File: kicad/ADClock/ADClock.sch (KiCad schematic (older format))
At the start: 26 parts, among them IC1 ATMEGA328-PU, IC2 ATMEGA328-PU, Y1 Crystal, Y2 Crystal

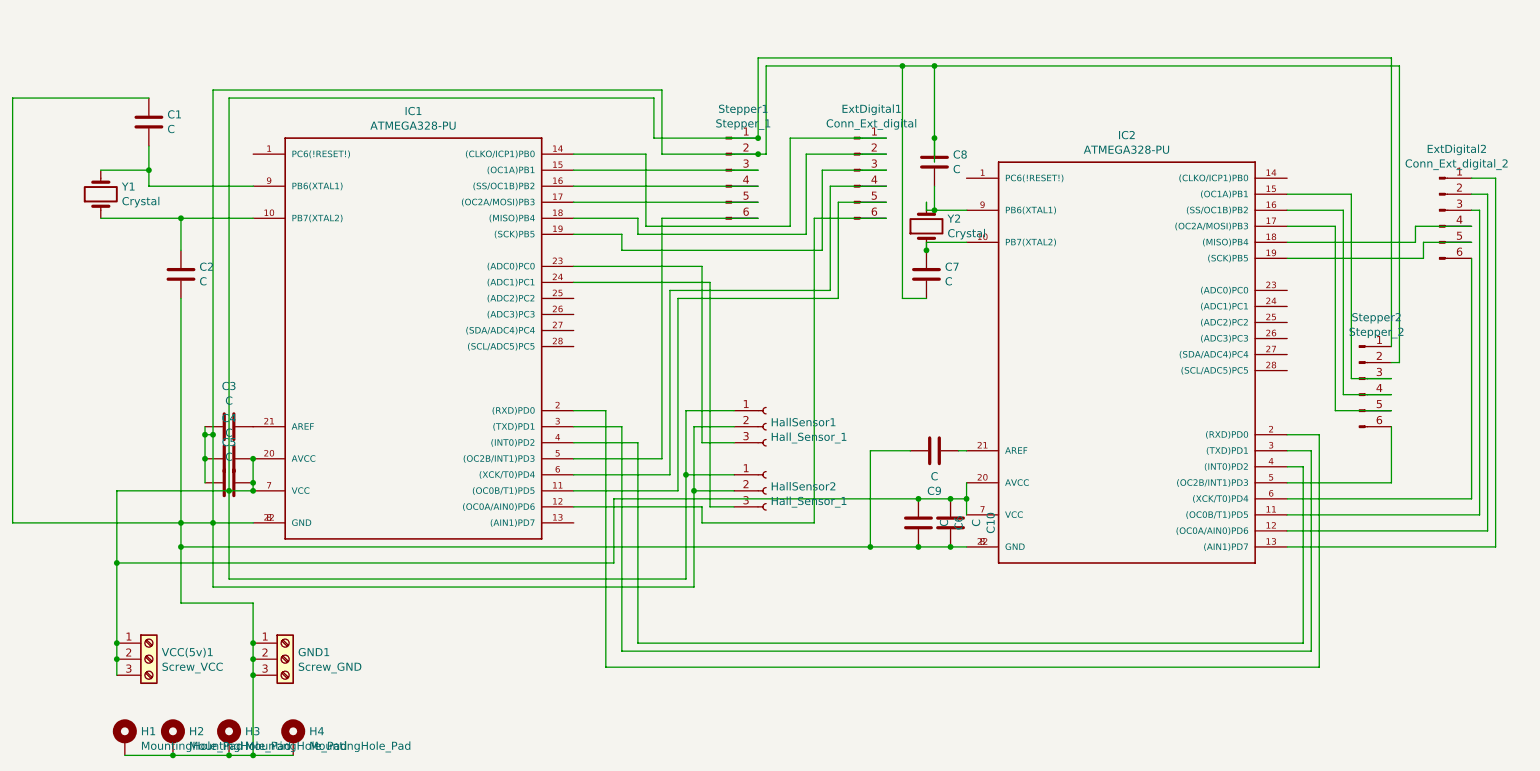
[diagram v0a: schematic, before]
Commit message: board changes
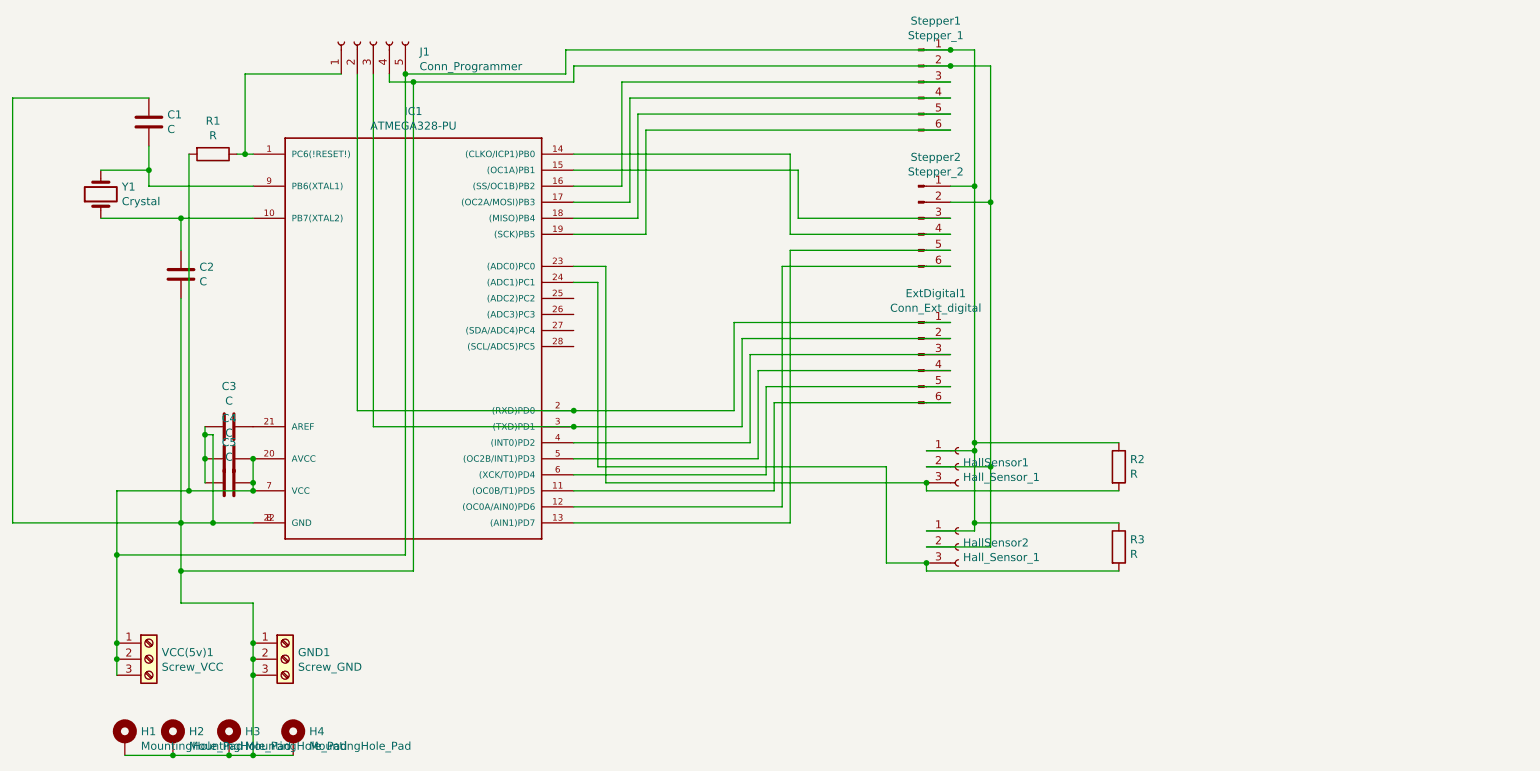
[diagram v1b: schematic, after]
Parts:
- removed C10, C6, C7, C8, C9: C, Capacitor_THT:C_Rect_L7.0mm_W2.5mm_P5.00mm, symbol Device:C
- removed ExtDigital2: Conn_Ext_digital_2, Connector_PinHeader_2.54mm:PinHeader_1x06_P2.54mm_Vertical, symbol Connector:Conn_01x06_Male
- removed IC2: ATMEGA328-PU, DIL28, symbol ATMEGA328-PU:ATMEGA328-PU
- removed Y2: Crystal, Crystal:Crystal_HC49-4H_Vertical, symbol Device:Crystal
- added J1: Conn_Programmer, Connector_PinHeader_2.54mm:PinHeader_1x05_P2.54mm_Vertical, symbol Connector:Conn_01x05_Female
- added R1, R2, R3: R, Resistor_THT:R_Axial_DIN0207_L6.3mm_D2.5mm_P7.62mm_Horizontal, symbol Device:R
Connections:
- net at C1.1, C2.2, C3.2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: now also J1.4 (Pin_4)
- net at IC1.1 (PC6(!RESET!)): now also J1.1 (Pin_1), R1.1
- net at IC1.11 ((OC0B/T1)PD5): now also ExtDigital1.6 (Pin_6); no longer ExtDigital1.5 (Pin_5)
- net at IC1.12 ((OC0A/AIN0)PD6): now also Stepper2.6 (Pin_6); no longer ExtDigital1.6 (Pin_6)
- net at IC1.13 ((AIN1)PD7): now also Stepper2.5 (Pin_5)
- net at IC1.14 ((CLKO/ICP1)PB0): now also Stepper2.4 (Pin_4); no longer ExtDigital1.1 (Pin_1)
- net at IC1.15 ((OC1A)PB1): now also Stepper2.3 (Pin_3); no longer Stepper1.3 (Pin_3)
- net at IC1.16 ((SS/OC1B)PB2): now also Stepper1.3 (Pin_3); no longer Stepper1.4 (Pin_4)
- net at IC1.17 ((OC2A/MOSI)PB3): now also Stepper1.4 (Pin_4); no longer Stepper1.5 (Pin_5)
- net at IC1.18 ((MISO)PB4): now also Stepper1.5 (Pin_5); no longer ExtDigital1.2 (Pin_2)
- net at IC1.19 ((SCK)PB5): now also Stepper1.6 (Pin_6); no longer ExtDigital1.3 (Pin_3)
- net at IC1.2 ((RXD)PD0): now also ExtDigital1.1 (Pin_1), J1.2 (Pin_2)
- net at C4.1, C5.2, HallSensor1.1 (Pin_1)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: now also J1.5 (Pin_5), R1.2, R2.1, R3.1
- net at HallSensor1.3 (Pin_3), IC1.23 ((ADC0)PC0): now also R2.2
- net at HallSensor2.3 (Pin_3), IC1.24 ((ADC1)PC1): now also R3.2
- net at IC1.3 ((TXD)PD1): now also ExtDigital1.2 (Pin_2), J1.3 (Pin_3)
- net at IC1.4 ((INT0)PD2): now also ExtDigital1.3 (Pin_3)
- net at IC1.5 ((OC2B/INT1)PD3): now also ExtDigital1.4 (Pin_4); no longer Stepper1.6 (Pin_6)
- net at IC1.6 ((XCK/T0)PD4): now also ExtDigital1.5 (Pin_5); no longer ExtDigital1.4 (Pin_4)
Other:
- moved on the sheet: ExtDigital1, HallSensor1, HallSensor2, Stepper1
